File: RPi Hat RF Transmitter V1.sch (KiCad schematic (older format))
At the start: 83 parts, among them CON1 Sig_In, CON2 SMA-, IC1 ADG904BRUZ-R, IC3 SN74HC139PW, IC4 ADG904BRUZ-R, J1 Conn_02x03_Odd_Even, J10 U.FL-R-SMT(10), J11 U.FL-R-SMT(10), J12 U.FL-R-SMT(10), J3 40HAT, J4 USB_B_Micro, J5 Conn_01x03_Male, J7 Conn_01x03_Male, J9 U.FL-R-SMT(10), U1 SBB5089Z, U2 LM1117-ADJ, U3 74AUC2G04, X1 C, X10 L, X2 L, X3 C, X4 L, X5 C, X6 L, X7 C, X8 L, X9 C

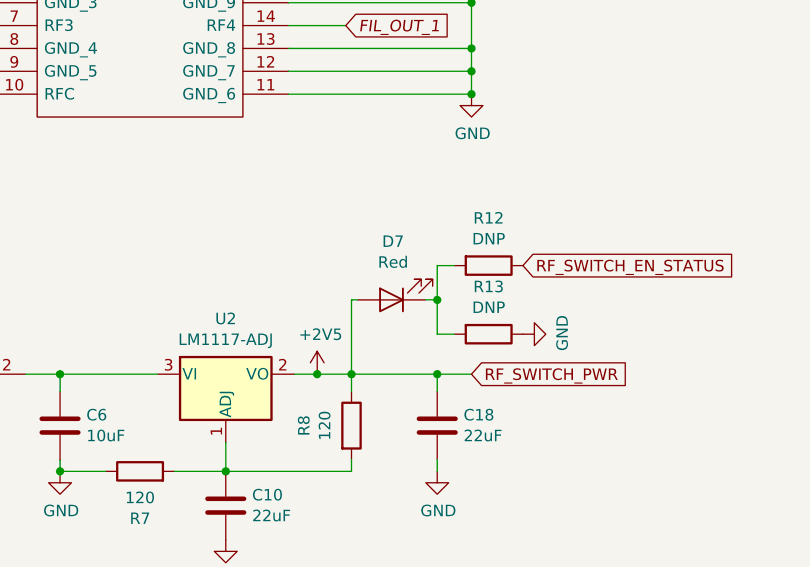
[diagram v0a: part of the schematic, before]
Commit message: adds silk screen updates, ground stiching and generated GERBERs
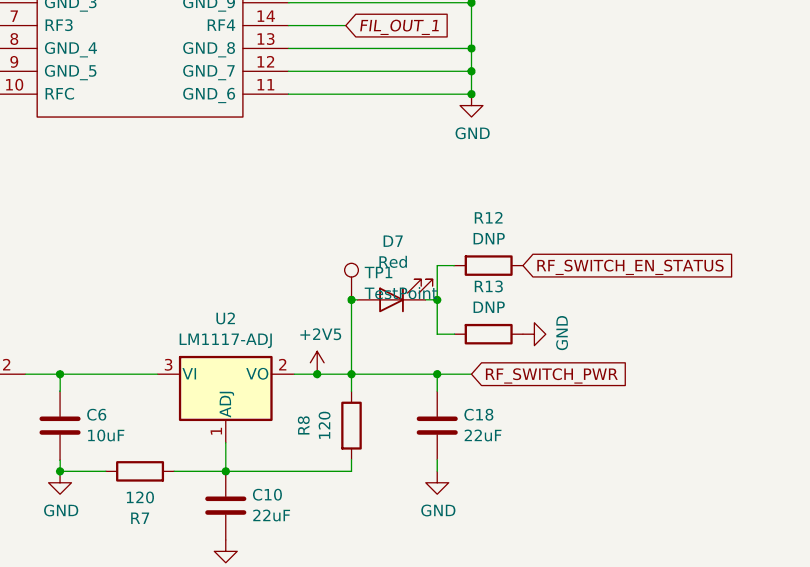
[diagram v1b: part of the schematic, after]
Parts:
- added TP1: TestPoint, Connector_Pin:Pin_D0.9mm_L10.0mm_W2.4mm_FlatFork, symbol Connector:TestPoint
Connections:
- net +2V5: now also TP1.1
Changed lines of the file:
@@
 Wire Wire Line
 	13375 2050 13550 2050
+$Comp
+L Connector:TestPoint TP1
+U 1 1 5DC2EB13
+P 13650 3850
+F 0 "TP1" H 13708 3968 50  0000 L CNN
+F 1 "TestPoint" H 13708 3877 50  0000 L CNN
+F 2 "Connector_Pin:Pin_D0.9mm_L10.0mm_W2.4mm_FlatFork" H 13850 3850 50  0001 C CNN
+F 3 "~" H 13850 3850 50  0001 C CNN
+	1    13650 3850
+	1    0    0    -1
+$EndComp
+Connection ~ 13650 3850
 $EndSCHEMATC
